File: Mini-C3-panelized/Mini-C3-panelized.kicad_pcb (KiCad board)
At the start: 2 copper layers, 98.1 x 91.9 mm, 194 parts, among them J1 TB_1X2, J10 Sensor1, J11 Sensor1, J12 Sensor1, J2 Sensor1, J3 Sensor1, J4 MotorB, J5 MotorA, J6 Sensor1, J7 Sensor1, J8 Sensor1, J9 Sensor1, SW1 SW_Push, SW2 SW_Push, SW3 SW_DIP_x02, U1 Driver Module, U2 ESP32-C3_SUPERMINI, U3 Mini360

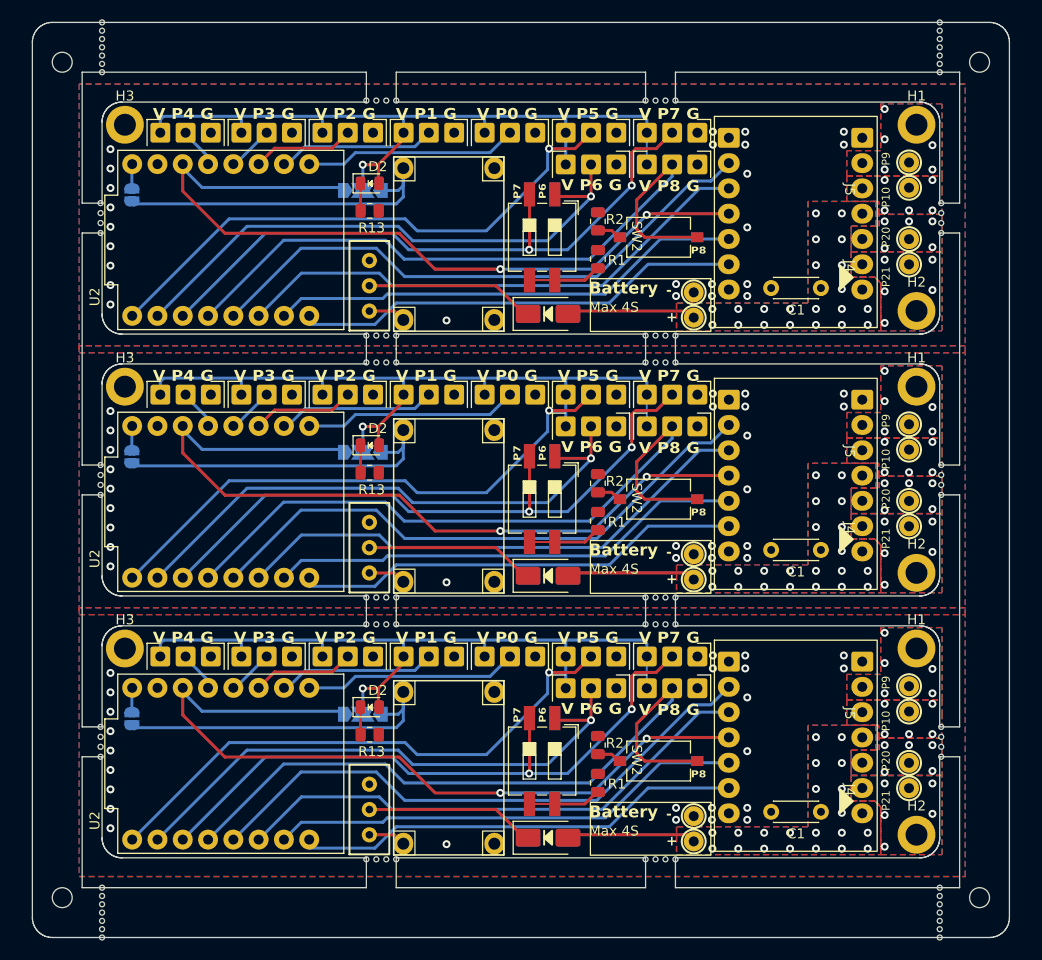
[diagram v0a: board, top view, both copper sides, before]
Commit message: panels
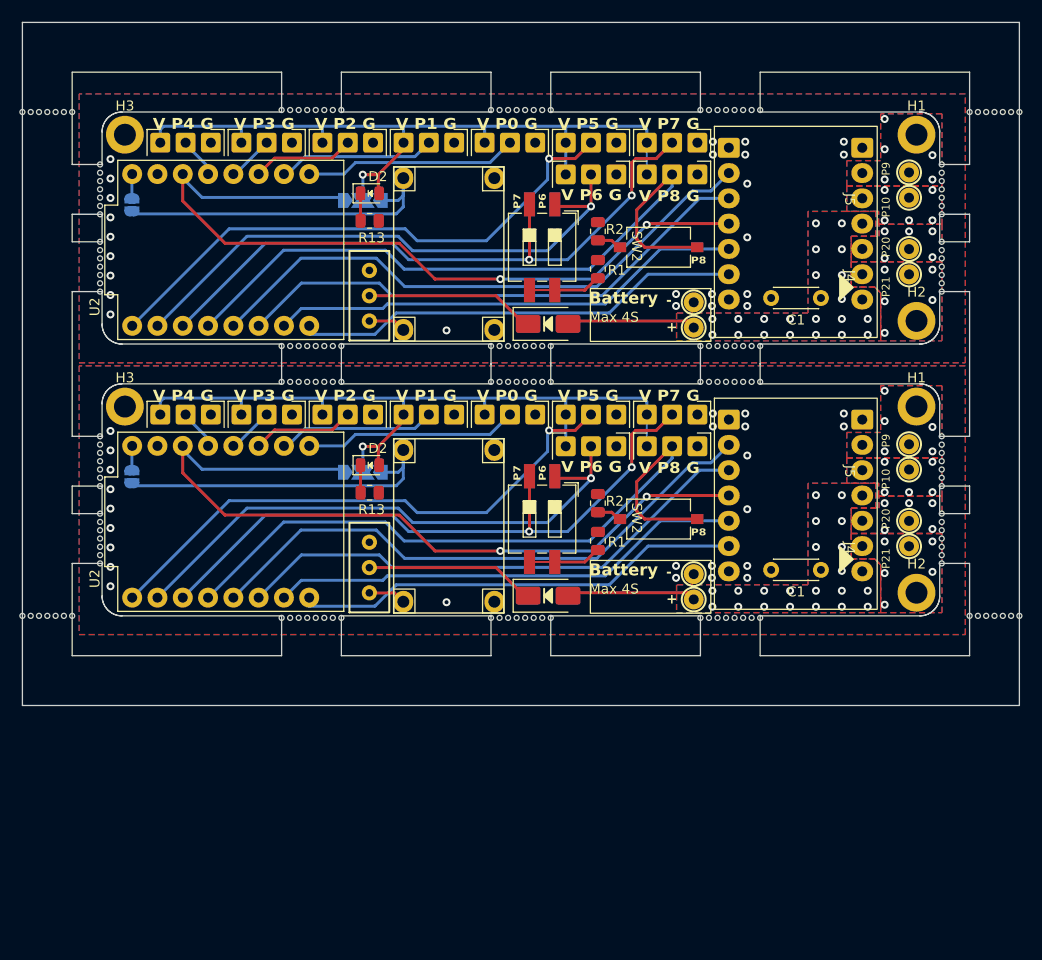
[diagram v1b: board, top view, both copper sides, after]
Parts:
- removed the C1 at (178.6, 73.0)
- removed the C1 at (178.6, 46.7)
- removed the C1 at (178.6, 99.3)
- removed the D1 at (151.2, 101.9)
- removed the D1 at (151.2, 49.3)
- removed the D1 at (151.2, 75.6)
- removed the D2 at (133.2, 88.8)
- removed the D2 at (133.2, 36.2)
- removed the D2 at (133.2, 62.5)
- removed the G*** at (157.0, 95.0)
- removed the G*** at (157.0, 42.4)
- removed the G*** at (157.0, 68.7)
- removed the H1 at (188.2, 82.9)
- removed the H1 at (188.2, 30.3)
- removed the H1 at (188.2, 56.6)
- removed the H2 at (188.2, 49.0)
- removed the H2 at (188.2, 101.6)
- removed the H2 at (188.2, 75.3)
- removed the H3 at (108.7, 30.3)
- removed the H3 at (108.7, 82.9)
- removed the H3 at (108.7, 56.6)
- removed the J1 at (161.1, 101.0)
- removed the J1 at (161.1, 74.7)
- removed the J1 at (161.1, 48.4)
- removed the J10 at (147.4, 84.4)
- removed the J10 at (147.4, 58.1)
- removed the J10 at (147.4, 31.8)
- removed the J11 at (163.7, 87.6)
- removed the J11 at (163.7, 61.3)
- removed the J11 at (163.7, 35.0)
- removed the J12 at (163.7, 84.4)
- removed the J12 at (163.7, 58.1)
- removed the J12 at (163.7, 31.8)
- removed the J2 at (155.5, 58.1)
- removed the J2 at (155.5, 84.4)
- removed the J2 at (155.5, 31.8)
- removed the J3 at (155.5, 61.3)
- removed the J3 at (155.5, 87.6)
- removed the J3 at (155.5, 35.0)
- removed the J4 at (187.5, 95.6)
- removed the J4 at (187.5, 43.0)
- removed the J4 at (187.5, 69.3)
- removed the J5 at (187.5, 87.9)
- removed the J5 at (187.5, 35.3)
- removed the J5 at (187.5, 61.6)
- removed the J6 at (139.3, 58.1)
- removed the J6 at (139.3, 84.4)
- removed the J6 at (139.3, 31.8)
- removed the J7 at (131.1, 31.8)
- removed the J7 at (131.1, 58.1)
- removed the J7 at (131.1, 84.4)
- removed the J8 at (123.0, 31.8)
- removed the J8 at (123.0, 58.1)
- removed the J8 at (123.0, 84.4)
- removed the J9 at (114.8, 31.8)
- removed the J9 at (114.8, 58.1)
- removed the J9 at (114.8, 84.4)
- removed the JP1 at (132.6, 36.9)
- removed the JP1 at (132.6, 63.2)
- removed the JP1 at (132.6, 89.5)
- removed the JP7 at (109.4, 37.3)
- removed the JP7 at (109.4, 63.6)
- removed the JP7 at (109.4, 89.9)
- removed KiKit_TO_1, KiKit_TO_2, KiKit_TO_3, KiKit_TO_4: NPTH, NPTH
- removed the R1 at (156.2, 40.0)
- removed the R1 at (156.2, 92.6)
- removed the R1 at (156.2, 66.3)
- removed the R13 at (133.3, 65.2)
- removed the R13 at (133.3, 91.5)
- removed the R13 at (133.3, 38.9)
- removed the R2 at (156.2, 70.1)
- removed the R2 at (156.2, 43.8)
- removed the R2 at (156.2, 96.4)
- removed the SW1 at (133.3, 72.8)
- removed the SW1 at (133.3, 99.0)
- removed the SW1 at (133.3, 46.5)
- removed the SW2 at (162.3, 67.9)
- removed the SW2 at (162.3, 41.6)
- removed the SW2 at (162.3, 94.2)
- removed the SW3 at (150.6, 41.6)
- removed the SW3 at (150.6, 67.9)
- removed the SW3 at (150.6, 94.2)
- removed the U1 at (176.0, 66.2)
- removed the U1 at (176.0, 39.9)
- removed the U1 at (176.0, 92.5)
- removed the U2 at (119.4, 68.2)
- removed the U2 at (119.4, 94.5)
- removed the U2 at (119.4, 41.9)
- removed the U3 at (141.3, 42.3)
- removed the U3 at (141.3, 94.9)
- removed the U3 at (141.3, 68.6)
- added C1: 100, Capacitor_THT:C_Disc_D4.3mm_W1.9mm_P5.00mm, F.Cu at (178.6, 75.0)
- added C1: 100, Capacitor_THT:C_Disc_D4.3mm_W1.9mm_P5.00mm, F.Cu at (178.6, 47.7)
- added D1: M7, Diode_SMD:D_SMA, F.Cu at (151.2, 50.3)
- added D1: M7, Diode_SMD:D_SMA, F.Cu at (151.2, 77.6)
- added D2: LED, MixLib:LED_0805_2012Metric, F.Cu at (133.2, 37.2)
- added D2: LED, MixLib:LED_0805_2012Metric, F.Cu at (133.2, 64.5)
- added G***: LOGO, LOGO, B.Cu at (157.0, 43.4)
- added G***: LOGO, LOGO, B.Cu at (157.0, 70.7)
- added H1: MountingHole_Pad, MountingHole:MountingHole_2.2mm_M2_DIN965_Pad, F.Cu at (188.2, 31.3)
- added H1: MountingHole_Pad, MountingHole:MountingHole_2.2mm_M2_DIN965_Pad, F.Cu at (188.2, 58.6)
- added H2: MountingHole_Pad, MountingHole:MountingHole_2.2mm_M2_DIN965_Pad, F.Cu at (188.2, 77.3)
- added H2: MountingHole_Pad, MountingHole:MountingHole_2.2mm_M2_DIN965_Pad, F.Cu at (188.2, 50.0)
- added H3: MountingHole_Pad, MountingHole:MountingHole_2.2mm_M2_DIN965_Pad, F.Cu at (108.7, 58.6)
- added H3: MountingHole_Pad, MountingHole:MountingHole_2.2mm_M2_DIN965_Pad, F.Cu at (108.7, 31.3)
- added J1: TB_1X2, MixLib:MyPinHeader-01x02-vertical, F.Cu at (161.1, 76.7)
- added J1: TB_1X2, MixLib:MyPinHeader-01x02-vertical, F.Cu at (161.1, 49.4)
- added J10: Sensor1, MixLib:PinHeader_1x03_P2.54-THT, F.Cu at (147.4, 60.1)
- added J10: Sensor1, MixLib:PinHeader_1x03_P2.54-THT, F.Cu at (147.4, 32.8)
- added J11: Sensor1, MixLib:PinHeader_1x03_P2.54-THT, F.Cu at (163.7, 63.3)
- added J11: Sensor1, MixLib:PinHeader_1x03_P2.54-THT, F.Cu at (163.7, 36.0)
- added J12: Sensor1, MixLib:PinHeader_1x03_P2.54-THT, F.Cu at (163.7, 32.8)
- added J12: Sensor1, MixLib:PinHeader_1x03_P2.54-THT, F.Cu at (163.7, 60.1)
- added J2: Sensor1, MixLib:PinHeader_1x03_P2.54-THT, F.Cu at (155.5, 60.1)
- added J2: Sensor1, MixLib:PinHeader_1x03_P2.54-THT, F.Cu at (155.5, 32.8)
- added J3: Sensor1, MixLib:PinHeader_1x03_P2.54-THT, F.Cu at (155.5, 63.3)
- added J3: Sensor1, MixLib:PinHeader_1x03_P2.54-THT, F.Cu at (155.5, 36.0)
- added J4: MotorB, MixLib:MyPinHeader-01x02, F.Cu at (187.5, 44.0)
- added J4: MotorB, MixLib:MyPinHeader-01x02, F.Cu at (187.5, 71.3)
- added J5: MotorA, MixLib:MyPinHeader-01x02, F.Cu at (187.5, 36.3)
- added J5: MotorA, MixLib:MyPinHeader-01x02, F.Cu at (187.5, 63.6)
- added J6: Sensor1, MixLib:PinHeader_1x03_P2.54-THT, F.Cu at (139.3, 60.1)
- added J6: Sensor1, MixLib:PinHeader_1x03_P2.54-THT, F.Cu at (139.3, 32.8)
- added J7: Sensor1, MixLib:PinHeader_1x03_P2.54-THT, F.Cu at (131.1, 60.1)
- added J7: Sensor1, MixLib:PinHeader_1x03_P2.54-THT, F.Cu at (131.1, 32.8)
- added J8: Sensor1, MixLib:PinHeader_1x03_P2.54-THT, F.Cu at (123.0, 60.1)
- added J8: Sensor1, MixLib:PinHeader_1x03_P2.54-THT, F.Cu at (123.0, 32.8)
- added J9: Sensor1, MixLib:PinHeader_1x03_P2.54-THT, F.Cu at (114.8, 32.8)
- added J9: Sensor1, MixLib:PinHeader_1x03_P2.54-THT, F.Cu at (114.8, 60.1)
- added JP1: Sensors voltage jumper, Jumper:SolderJumper-3_P2.0mm_Open_TrianglePad1.0x1.5mm, B.Cu at (132.6, 37.9)
- added JP1: Sensors voltage jumper, Jumper:SolderJumper-3_P2.0mm_Open_TrianglePad1.0x1.5mm, B.Cu at (132.6, 65.2)
- added JP7: Jumper_2_Small_Open, Jumper:SolderJumper-2_P1.3mm_Open_RoundedPad1.0x1.5mm, B.Cu at (109.4, 38.3)
- added JP7: Jumper_2_Small_Open, Jumper:SolderJumper-2_P1.3mm_Open_RoundedPad1.0x1.5mm, B.Cu at (109.4, 65.6)
- added KiKit_MB_10_5: NPTH, NPTH, F.Cu at (169.1, 52.5)
- added KiKit_MB_10_6: NPTH, NPTH, F.Cu at (168.2, 52.5)
- added KiKit_MB_10_7: NPTH, NPTH, F.Cu at (167.4, 52.5)
- added KiKit_MB_10_8: NPTH, NPTH, F.Cu at (166.5, 52.5)
- added KiKit_MB_11_5: NPTH, NPTH, F.Cu at (106.2, 63.2)
- added KiKit_MB_11_6: NPTH, NPTH, F.Cu at (106.2, 62.4)
- added KiKit_MB_11_7: NPTH, NPTH, F.Cu at (106.2, 61.6)
- added KiKit_MB_12_5: NPTH, NPTH, F.Cu at (106.2, 71.0)
- added KiKit_MB_12_6: NPTH, NPTH, F.Cu at (106.2, 70.2)
- added KiKit_MB_12_7: NPTH, NPTH, F.Cu at (106.2, 69.3)
- added KiKit_MB_13_5: NPTH, NPTH, F.Cu at (190.8, 64.9)
- added KiKit_MB_13_6: NPTH, NPTH, F.Cu at (190.8, 65.7)
- added KiKit_MB_13_7: NPTH, NPTH, F.Cu at (190.8, 66.6)
- added KiKit_MB_14_5: NPTH, NPTH, F.Cu at (190.8, 72.7)
- added KiKit_MB_14_6: NPTH, NPTH, F.Cu at (190.8, 73.5)
- added KiKit_MB_14_7: NPTH, NPTH, F.Cu at (190.8, 74.3)
- added KiKit_MB_15_5: NPTH, NPTH, F.Cu at (127.9, 56.1)
- added KiKit_MB_15_6: NPTH, NPTH, F.Cu at (128.8, 56.1)
- added KiKit_MB_15_7: NPTH, NPTH, F.Cu at (129.6, 56.1)
- added KiKit_MB_15_8: NPTH, NPTH, F.Cu at (130.5, 56.1)
- added KiKit_MB_16_5: NPTH, NPTH, F.Cu at (148.9, 56.1)
- added KiKit_MB_16_6: NPTH, NPTH, F.Cu at (149.8, 56.1)
- added KiKit_MB_16_7: NPTH, NPTH, F.Cu at (150.6, 56.1)
- added KiKit_MB_16_8: NPTH, NPTH, F.Cu at (151.5, 56.1)
- added KiKit_MB_17_5: NPTH, NPTH, F.Cu at (170.0, 56.1)
- added KiKit_MB_17_6: NPTH, NPTH, F.Cu at (170.8, 56.1)
- added KiKit_MB_17_7: NPTH, NPTH, F.Cu at (171.7, 56.1)
- added KiKit_MB_17_8: NPTH, NPTH, F.Cu at (172.5, 56.1)
- added KiKit_MB_18_5: NPTH, NPTH, F.Cu at (127.0, 79.8)
- added KiKit_MB_18_6: NPTH, NPTH, F.Cu at (126.2, 79.8)
- added KiKit_MB_18_7: NPTH, NPTH, F.Cu at (125.3, 79.8)
- added KiKit_MB_18_8: NPTH, NPTH, F.Cu at (124.5, 79.8)
- added KiKit_MB_19_8: NPTH, NPTH, F.Cu at (145.5, 79.8)
- added KiKit_MB_1_5: NPTH, NPTH, F.Cu at (106.2, 35.9)
- added KiKit_MB_1_6: NPTH, NPTH, F.Cu at (106.2, 35.1)
- added KiKit_MB_1_7: NPTH, NPTH, F.Cu at (106.2, 34.3)
- added KiKit_MB_20_8: NPTH, NPTH, F.Cu at (166.5, 79.8)
- added KiKit_MB_23_1: NPTH, NPTH, F.Cu at (193.6, 29.0)
- added KiKit_MB_23_2: NPTH, NPTH, F.Cu at (194.4, 29.0)
- added KiKit_MB_23_3: NPTH, NPTH, F.Cu at (195.2, 29.0)
- added KiKit_MB_23_4: NPTH, NPTH, F.Cu at (196.1, 29.0)
- added KiKit_MB_23_5: NPTH, NPTH, F.Cu at (196.9, 29.0)
- added KiKit_MB_23_6: NPTH, NPTH, F.Cu at (197.7, 29.0)
- added KiKit_MB_23_7: NPTH, NPTH, F.Cu at (198.6, 29.0)
- added KiKit_MB_24_1: NPTH, NPTH, F.Cu at (193.6, 79.6)
- added KiKit_MB_24_2: NPTH, NPTH, F.Cu at (194.4, 79.6)
- added KiKit_MB_24_3: NPTH, NPTH, F.Cu at (195.2, 79.6)
- added KiKit_MB_24_4: NPTH, NPTH, F.Cu at (196.1, 79.6)
- added KiKit_MB_24_5: NPTH, NPTH, F.Cu at (196.9, 79.6)
- added KiKit_MB_24_6: NPTH, NPTH, F.Cu at (197.7, 79.6)
- added KiKit_MB_24_7: NPTH, NPTH, F.Cu at (198.6, 79.6)
- added KiKit_MB_2_5: NPTH, NPTH, F.Cu at (106.2, 43.7)
- added KiKit_MB_2_6: NPTH, NPTH, F.Cu at (106.2, 42.9)
- added KiKit_MB_2_7: NPTH, NPTH, F.Cu at (106.2, 42.0)
- added KiKit_MB_3_5: NPTH, NPTH, F.Cu at (190.8, 37.6)
- added KiKit_MB_3_6: NPTH, NPTH, F.Cu at (190.8, 38.4)
- added KiKit_MB_3_7: NPTH, NPTH, F.Cu at (190.8, 39.3)
- added KiKit_MB_4_5: NPTH, NPTH, F.Cu at (190.8, 45.4)
- added KiKit_MB_4_6: NPTH, NPTH, F.Cu at (190.8, 46.2)
- added KiKit_MB_4_7: NPTH, NPTH, F.Cu at (190.8, 47.0)
- added KiKit_MB_5_5: NPTH, NPTH, F.Cu at (127.9, 28.8)
- added KiKit_MB_5_6: NPTH, NPTH, F.Cu at (128.8, 28.8)
- added KiKit_MB_5_7: NPTH, NPTH, F.Cu at (129.6, 28.8)
- added KiKit_MB_5_8: NPTH, NPTH, F.Cu at (130.5, 28.8)
- added KiKit_MB_6_5: NPTH, NPTH, F.Cu at (148.9, 28.8)
- added KiKit_MB_6_6: NPTH, NPTH, F.Cu at (149.8, 28.8)
- added KiKit_MB_6_7: NPTH, NPTH, F.Cu at (150.6, 28.8)
- added KiKit_MB_6_8: NPTH, NPTH, F.Cu at (151.5, 28.8)
- added KiKit_MB_7_5: NPTH, NPTH, F.Cu at (170.0, 28.8)
- added KiKit_MB_7_6: NPTH, NPTH, F.Cu at (170.8, 28.8)
- added KiKit_MB_7_7: NPTH, NPTH, F.Cu at (171.7, 28.8)
- added KiKit_MB_7_8: NPTH, NPTH, F.Cu at (172.5, 28.8)
- added KiKit_MB_8_5: NPTH, NPTH, F.Cu at (127.0, 52.5)
- added KiKit_MB_8_6: NPTH, NPTH, F.Cu at (126.2, 52.5)
- added KiKit_MB_8_7: NPTH, NPTH, F.Cu at (125.3, 52.5)
- added KiKit_MB_8_8: NPTH, NPTH, F.Cu at (124.5, 52.5)
- added KiKit_MB_9_5: NPTH, NPTH, F.Cu at (148.1, 52.5)
- added KiKit_MB_9_6: NPTH, NPTH, F.Cu at (147.2, 52.5)
- added KiKit_MB_9_7: NPTH, NPTH, F.Cu at (146.4, 52.5)
- added KiKit_MB_9_8: NPTH, NPTH, F.Cu at (145.5, 52.5)
- added R1: 100, Resistor_SMD:R_0805_2012Metric, F.Cu at (156.2, 41.0)
- added R1: 100, Resistor_SMD:R_0805_2012Metric, F.Cu at (156.2, 68.3)
- added R13: 2,7k, Resistor_SMD:R_0805_2012Metric, F.Cu at (133.3, 67.2)
- added R13: 2,7k, Resistor_SMD:R_0805_2012Metric, F.Cu at (133.3, 39.9)
- added R2: 100, Resistor_SMD:R_0805_2012Metric, F.Cu at (156.2, 72.1)
- added R2: 100, Resistor_SMD:R_0805_2012Metric, F.Cu at (156.2, 44.8)
- added SW1: SW_Push, MixLib:SW_Slide-03_P2.54_L9_W4_H7, F.Cu at (133.3, 74.8)
- added SW1: SW_Push, MixLib:SW_Slide-03_P2.54_L9_W4_H7, F.Cu at (133.3, 47.5)
- added SW2: SW_Push, Button_Switch_SMD:SW_Tactile_SPST_NO_Straight_CK_PTS636Sx25SMTRLFS, F.Cu at (162.3, 69.9)
- added SW2: SW_Push, Button_Switch_SMD:SW_Tactile_SPST_NO_Straight_CK_PTS636Sx25SMTRLFS, F.Cu at (162.3, 42.6)
- added SW3: SW_DIP_x02, Button_Switch_SMD:SW_DIP_SPSTx02_Slide_6.7x6.64mm_W8.61mm_P2.54mm_LowProfile, F.Cu at (150.6, 69.9)
- added SW3: SW_DIP_x02, Button_Switch_SMD:SW_DIP_SPSTx02_Slide_6.7x6.64mm_W8.61mm_P2.54mm_LowProfile, F.Cu at (150.6, 42.6)
- added U1: Driver Module, MixLib:Dual-Driver-Module, F.Cu at (176.0, 68.2)
- added U1: Driver Module, MixLib:Dual-Driver-Module, F.Cu at (176.0, 40.9)
- added U2: ESP32-C3_SUPERMINI, MixLib:MODULE_ESP32-C3_SUPERMINI, F.Cu at (119.4, 70.2)
- added U2: ESP32-C3_SUPERMINI, MixLib:MODULE_ESP32-C3_SUPERMINI, F.Cu at (119.4, 42.9)
- added U3: Mini360, MixLib:Mini360_step-down, F.Cu at (141.3, 43.3)
- added U3: Mini360, MixLib:Mini360_step-down, F.Cu at (141.3, 70.6)
- moved KiKit_MB_22_1 96.1 mm to (98.4, 79.6)
- moved KiKit_MB_22_2 95.5 mm to (99.3, 79.6)
- moved KiKit_MB_22_3 95.0 mm to (100.1, 79.6)
- moved KiKit_MB_22_4 94.4 mm to (100.9, 79.6)
- moved KiKit_MB_22_5 93.9 mm to (101.8, 79.6)
- moved KiKit_MB_22_6 93.4 mm to (102.6, 79.6)
- moved KiKit_MB_22_7 92.9 mm to (103.4, 79.6)
- moved KiKit_MB_13_1 90.4 mm to (190.8, 61.6)
- moved KiKit_MB_13_2 89.8 mm to (190.8, 62.4)
- moved KiKit_MB_13_3 89.2 mm to (190.8, 63.2)
- moved KiKit_MB_13_4 88.6 mm to (190.8, 64.1)
- moved KiKit_MB_2_1 84.9 mm to (106.2, 47.0)
- moved KiKit_MB_2_2 84.8 mm to (106.2, 46.2)
- moved KiKit_MB_2_3 84.6 mm to (106.2, 45.4)
- moved KiKit_MB_2_4 84.5 mm to (106.2, 44.5)
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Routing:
- net Board_2-+3.3V: track 80.4 -> 0.00 mm, vias 2 -> 0
- net Board_2-/Vcc: track 76.5 -> 0.00 mm, vias 1 -> 0
- net Board_2-/Pin8: track 69.6 -> 0.00 mm
- net Board_2-/Pin7: track 65.6 -> 0.00 mm, vias 2 -> 0
- net Board_2-/IN_B2: track 58.5 -> 0.00 mm
- net Board_2-/Pin6: track 56.7 -> 0.00 mm, vias 1 -> 0
- net Board_2-/Pin5: track 55.8 -> 0.00 mm, vias 1 -> 0
- net Board_2-/IN_B1: track 53.6 -> 0.00 mm
- net Board_2-/IN_A2: track 47.9 -> 0.00 mm
- net Board_2-/IN_A1: track 45.5 -> 0.00 mm
- net Board_2-+5V: track 34.5 -> 0.00 mm
- net Board_2-/Pin0: track 21.5 -> 0.00 mm
- net Board_2-Net-(D1-K): track 17.0 -> 0.00 mm
- net Board_2-/Pin1: track 15.9 -> 0.00 mm
- net Board_2-/VM: track 12.9 -> 0.00 mm, vias 21 -> 0
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- removed copper zone on B.Cu, net Board_2-/OUT_A1
- removed copper zone on F.Cu, net Board_2-/OUT_A1
- removed copper zone on B.Cu, net Board_2-/OUT_A2
- removed copper zone on F.Cu, net Board_2-/OUT_A2
- removed copper zone on B.Cu, net Board_2-/OUT_B1
- removed copper zone on F.Cu, net Board_2-/OUT_B1
- removed copper zone on B.Cu, net Board_2-/OUT_B2
- removed copper zone on F.Cu, net Board_2-/OUT_B2
- removed copper zone on B.Cu, net Board_2-/VM
- removed copper zone on F.Cu, net Board_2-/VM
- removed copper zone on B.Cu, net Board_2-GND
- removed copper zone on F.Cu, net Board_2-GND
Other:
- board size 98.1 x 91.9 mm -> 100.1 x 68.6 mm
